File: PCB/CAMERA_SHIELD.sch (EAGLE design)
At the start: 73 parts, among them IC4 LSF0204PWR, J1 47346-0001, Q1 FDN304P, Q2 FDN304P, Q3 SSM3J338R,LF, Q4 SSM3J338R,LF, Q5 FDN304P, U1 LARA-R2

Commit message: smartcamera with gsm
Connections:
- new net N$196: U1.VCC
- net V_GSM: no longer U1.VCC
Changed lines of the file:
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@@
 <net name="V_GSM" class="0">
+<segment>
+<junction x="223.73" y="282.65"/>
+<wire x1="223.73" y1="277.57" x2="223.73" y2="282.65" width="0.1524" layer="91"/>
+<pinref part="C24" gate="G$1" pin="1"/>
+</segment>
 <segment>
 <wire x1="223.8" y1="282.65" x2="233.89" y2="282.65" width="0.1524" layer="91"/>
@@
 <wire x1="254.21" y1="282.65" x2="264.37" y2="282.65" width="0.1524" layer="91"/>
 <wire x1="274.53" y1="282.65" x2="287.23" y2="282.65" width="0.1524" layer="91"/>
-<wire x1="223.73" y1="277.57" x2="223.73" y2="282.65" width="0.1524" layer="91"/>
-<junction x="223.73" y="282.65"/>
 <wire x1="233.89" y1="277.57" x2="233.89" y2="282.65" width="0.1524" layer="91"/>
 <junction x="233.89" y="282.65"/>
@@
 <pinref part="C15" gate="G$1" pin="1"/>
 <pinref part="C17" gate="G$1" pin="1"/>
-<pinref part="C24" gate="G$1" pin="1"/>
 <pinref part="V_GSM" gate="G$1" pin="TP"/>
 <pinref part="TVS8" gate="G$1" pin="2"/>
-<pinref part="U1" gate="G$1" pin="VCC"/>
-<wire x1="178.71" y1="282.65" x2="223.75" y2="282.65" width="0.1524" layer="91"/>
 <wire x1="223.8" y1="282.55" x2="223.8" y2="282.65" width="0.1524" layer="91"/>
-<wire x1="223.75" y1="282.65" x2="223.95" y2="282.65" width="0.1524" layer="91"/>
 <wire x1="223.95" y1="282.65" x2="223.95" y2="282.4" width="0.1524" layer="91"/>
 </segment>
@@
 </segment>
 </net>
+<net name="N$196" class="0">
+<segment>
+<pinref part="U1" gate="G$1" pin="VCC"/>
+<wire x1="178.71" y1="282.65" x2="223.75" y2="282.65" width="0.1524" layer="91"/>
+</segment>
+</net>

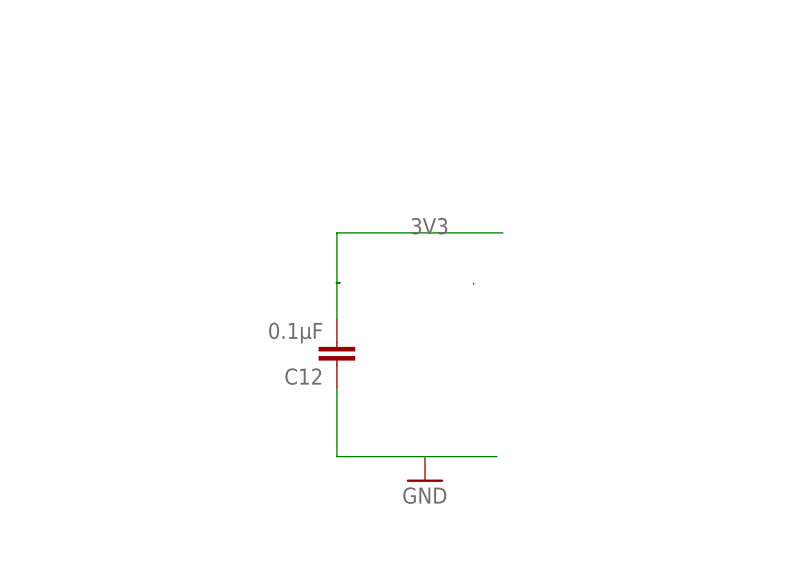
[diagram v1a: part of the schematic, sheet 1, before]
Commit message: fix router
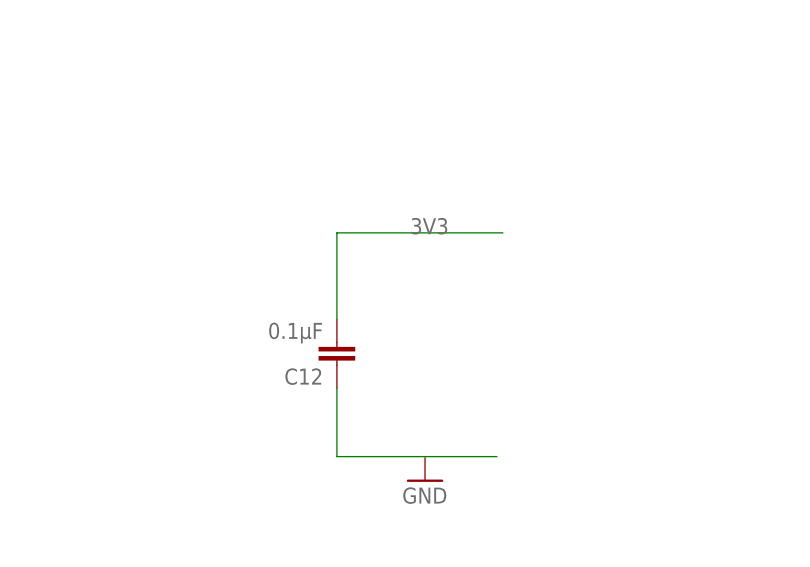
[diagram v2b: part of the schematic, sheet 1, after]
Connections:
- removed net N$196: U1.VCC
- net V_GSM: now also U1.VCC
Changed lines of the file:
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@@
-</segment>
-<segment>
-<wire x1="-54" y1="45.2" x2="-53.6" y2="45.2" width="0.1524" layer="91"/>
-<wire x1="-54" y1="45.15" x2="-54" y2="45.2" width="0.1524" layer="91"/>
-<wire x1="-53.95" y1="45.15" x2="-53.6" y2="45.2" width="0.1524" layer="91"/>
 </segment>
 <segment>
@@
 <pinref part="HUNG" gate="G$1" pin="PA15"/>
 <wire x1="128.53" y1="152.46" x2="128.53" y2="161.26" width="0.1524" layer="91"/>
-</segment>
-</net>
-<net name="N$10" class="0">
-<segment>
-<wire x1="-38.75" y1="45.15" x2="-38.75" y2="45.05" width="0.1524" layer="91"/>
 </segment>
 </net>
@@
 <pinref part="U1" gate="G$1" pin="V_INT"/>
 <wire x1="178.71" y1="277.57" x2="202.98" y2="277.57" width="0.1524" layer="91"/>
-<wire x1="202.98" y1="277.57" x2="202.98" y2="277.36" width="0.1524" layer="91"/>
 <label x="183.92" y="277.82" size="1.778" layer="95"/>
 </segment>
@@
 <pinref part="U1" gate="G$1" pin="V_BCKP"/>
 <wire x1="178.71" y1="280.11" x2="203.57" y2="280.11" width="0.1524" layer="91"/>
-<wire x1="203.57" y1="280.11" x2="203.57" y2="279.99" width="0.1524" layer="91"/>
 <label x="180.4" y="279.99" size="1.778" layer="95"/>
 </segment>
@@
 <net name="V_GSM" class="0">
 <segment>
-<junction x="223.73" y="282.65"/>
-<wire x1="223.73" y1="277.57" x2="223.73" y2="282.65" width="0.1524" layer="91"/>
-<pinref part="C24" gate="G$1" pin="1"/>
-</segment>
-<segment>
 <wire x1="223.8" y1="282.65" x2="233.89" y2="282.65" width="0.1524" layer="91"/>
 <wire x1="233.89" y1="282.65" x2="244.05" y2="282.65" width="0.1524" layer="91"/>
@@
 <wire x1="254.21" y1="282.65" x2="264.37" y2="282.65" width="0.1524" layer="91"/>
 <wire x1="274.53" y1="282.65" x2="287.23" y2="282.65" width="0.1524" layer="91"/>
+<wire x1="223.73" y1="277.57" x2="223.73" y2="282.65" width="0.1524" layer="91"/>
+<junction x="223.73" y="282.65"/>
 <wire x1="233.89" y1="277.57" x2="233.89" y2="282.65" width="0.1524" layer="91"/>
 <junction x="233.89" y="282.65"/>
@@
 <pinref part="C15" gate="G$1" pin="1"/>
 <pinref part="C17" gate="G$1" pin="1"/>
+<pinref part="C24" gate="G$1" pin="1"/>
 <pinref part="V_GSM" gate="G$1" pin="TP"/>
 <pinref part="TVS8" gate="G$1" pin="2"/>
+<pinref part="U1" gate="G$1" pin="VCC"/>
+<wire x1="178.71" y1="282.65" x2="223.75" y2="282.65" width="0.1524" layer="91"/>
 <wire x1="223.8" y1="282.55" x2="223.8" y2="282.65" width="0.1524" layer="91"/>
+<wire x1="223.75" y1="282.65" x2="223.95" y2="282.65" width="0.1524" layer="91"/>
 <wire x1="223.95" y1="282.65" x2="223.95" y2="282.4" width="0.1524" layer="91"/>
 </segment>
@@
 <label x="86.95" y="314.89" size="1.778" layer="95"/>
 </segment>
-<segment>
-<wire x1="203.22" y1="277.57" x2="203.22" y2="277.63" width="0.1524" layer="91"/>
-</segment>
 </net>
 <net name="GSM_EN" class="0">
@@
 </segment>
 </net>
-<net name="N$196" class="0">
-<segment>
-<pinref part="U1" gate="G$1" pin="VCC"/>
-<wire x1="178.71" y1="282.65" x2="223.75" y2="282.65" width="0.1524" layer="91"/>
-</segment>
-</net>
